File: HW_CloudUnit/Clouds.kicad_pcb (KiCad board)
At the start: 2 copper layers, 22 x 27 mm, 31 parts, among them J1 Conn_01x06, J2 Conn_01x04, J3 Conn_01x04, J4 Conn_01x04, U1 STM32G030F6Px, U2 AS5600L-ASOM, U3 DRV8313PWPR

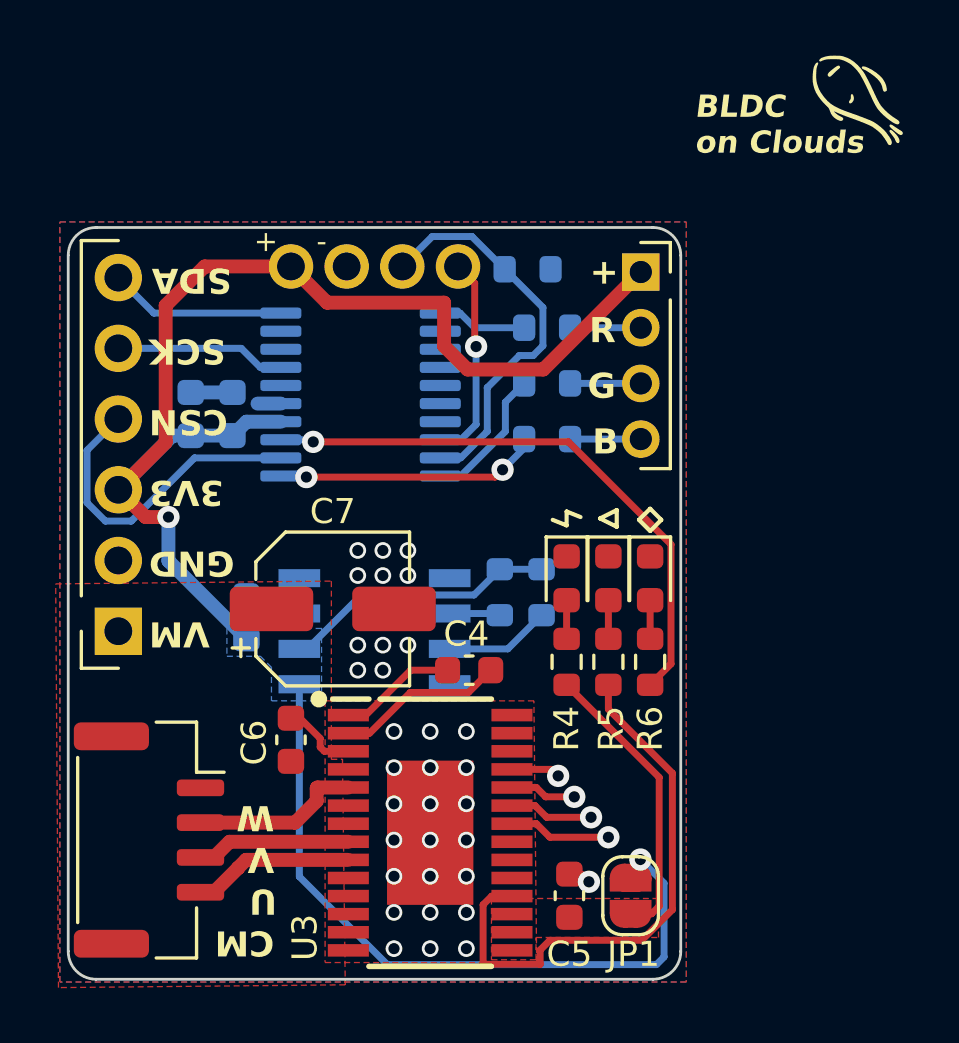
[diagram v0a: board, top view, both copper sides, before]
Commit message: Finish driver board design
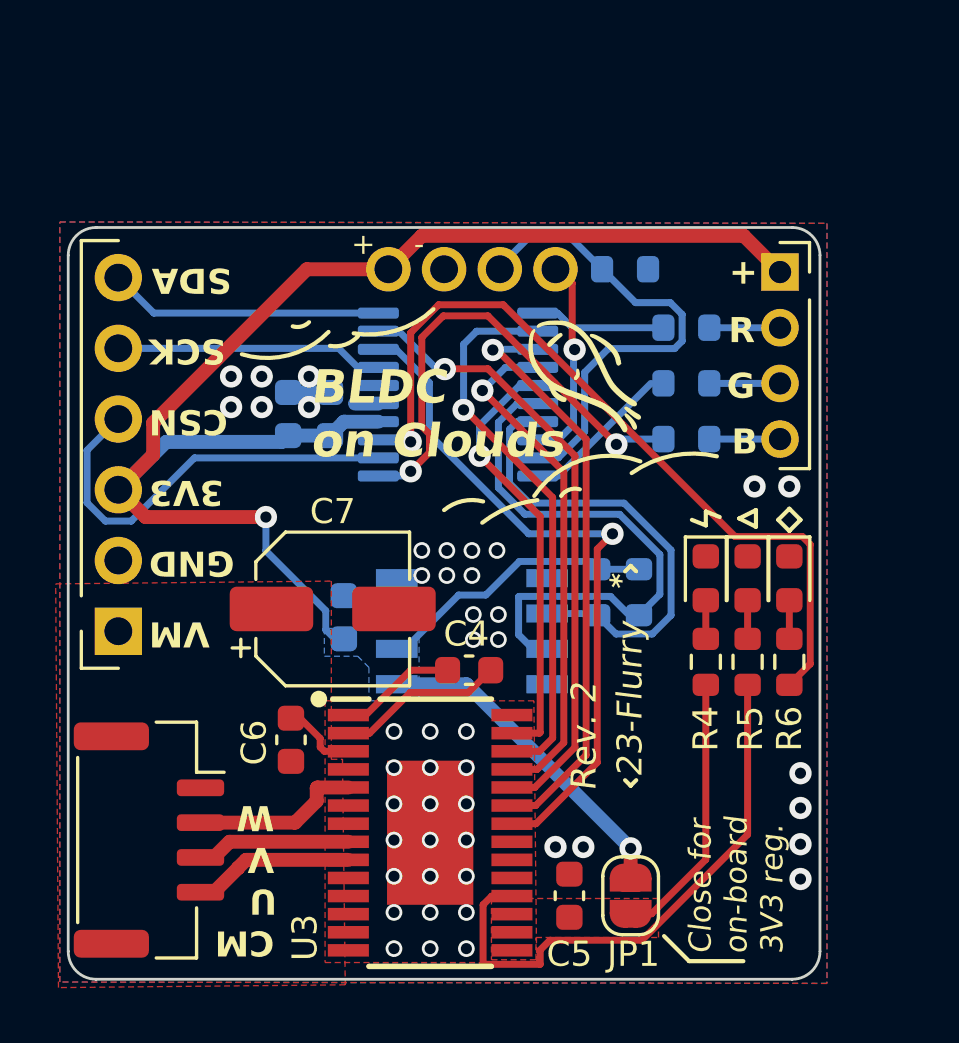
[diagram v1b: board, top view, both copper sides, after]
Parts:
- moved G*** 21.7 mm to (28.9, 43.9)
- moved G*** 21.7 mm to (21.2, 42.3)
- moved G*** 21.7 mm to (25.7, 42.6)
- moved G*** 13.9 mm to (36.8, 23.6)
- moved D1 5.00 mm to (41.1, 30.8)
- moved D2 5.00 mm to (42.6, 30.8)
- moved D3 5.00 mm to (44.1, 30.8)
- moved J3 5.00 mm to (43.8, 19.8)
- moved R4 5.00 mm to (41.1, 33.8)
- moved R5 5.00 mm to (42.6, 33.8)
- moved R6 5.00 mm to (44.1, 33.8)
- moved R7 5.00 mm to (40.4, 21.8)
- moved R8 5.00 mm to (40.4, 23.8)
- moved R9 5.00 mm to (40.4, 25.8)
- moved J4 3.50 mm to (32.7, 19.7)
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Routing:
- net EN_U: track 3.66 -> 24.7 mm
- net EN_W: track 0.00 -> 20.0 mm, vias 0 -> 1
- net EN_V: track 2.38 -> 22.3 mm
- net IN_U: track 3.01 -> 21.1 mm
- net MAG_SCL: track 3.80 -> 20.5 mm
- net IN_V: track 1.76 -> 18.5 mm
- net IN_W: track 0.00 -> 15.6 mm, vias 0 -> 1
- net MAG_SDA: track 1.82 -> 17.2 mm
- net LED_B: track 9.51 -> 17.4 mm
- net LED_ACT: track 20.9 -> 28.8 mm
- net +3.3V: track 79.6 -> 72.7 mm
- net UNIT_SCK: track 6.12 -> 9.62 mm
- net UNIT_SDA: track 6.37 -> 9.87 mm
- net UNIT_CSN: track 11.6 -> 15.1 mm
- net SWCLK: track 14.2 -> 17.2 mm
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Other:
- board size 22 x 27 mm -> 27 x 27 mm
- board text added: "BLDC (Y-wired) + Mag. Enc."
- board text added: "Close for on-board 3V3 reg."
- board text added: "In 8-50 V Out 1.75 A RMS"
- board text added: "Rev. 2"
- board text removed: "BLDC Driver (Y-wired) Magnet Encoder"
- board text removed: "Input 8-60 V Output 1.75 A RMS"
- board text removed: "Rev. 1"
